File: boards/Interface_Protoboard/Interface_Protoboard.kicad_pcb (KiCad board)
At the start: 2 copper layers, 70 x 70 mm, 385 parts

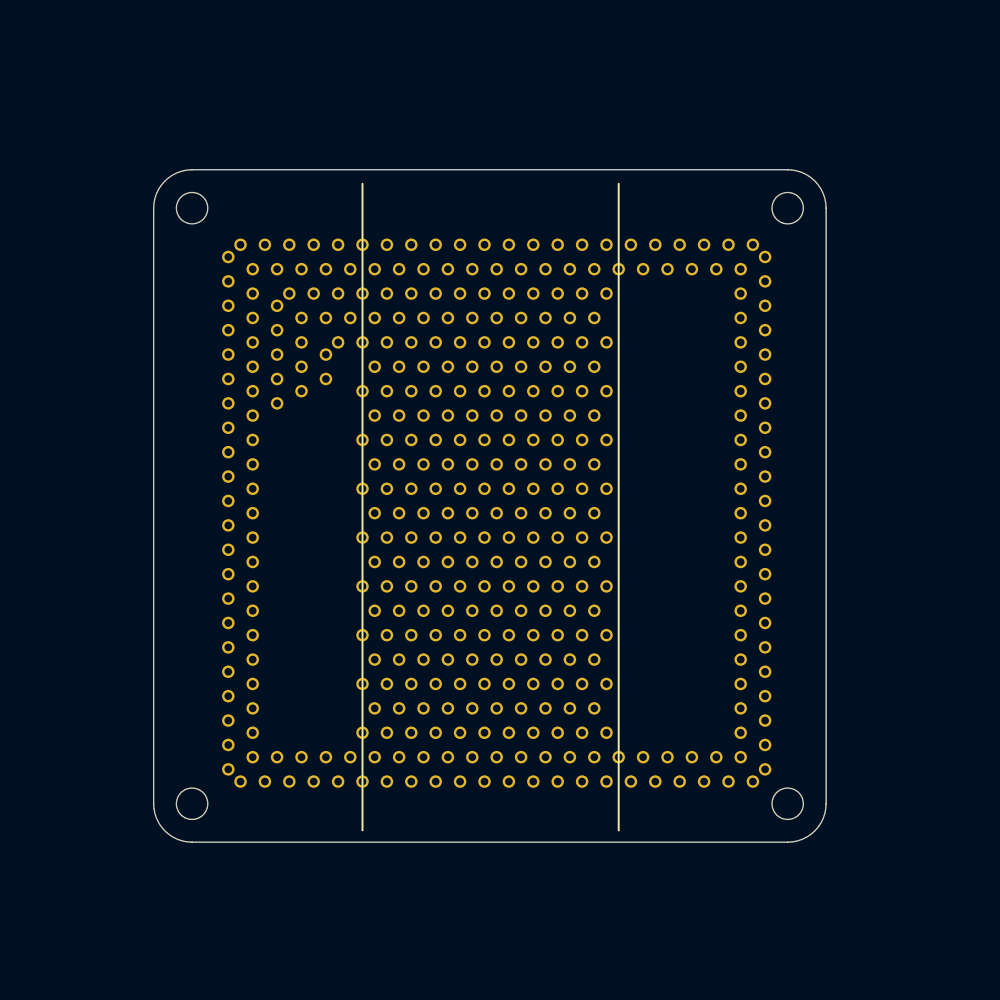
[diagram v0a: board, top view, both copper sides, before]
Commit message: finished interface protoboard and uploaded checked gerbers to drive for ordering
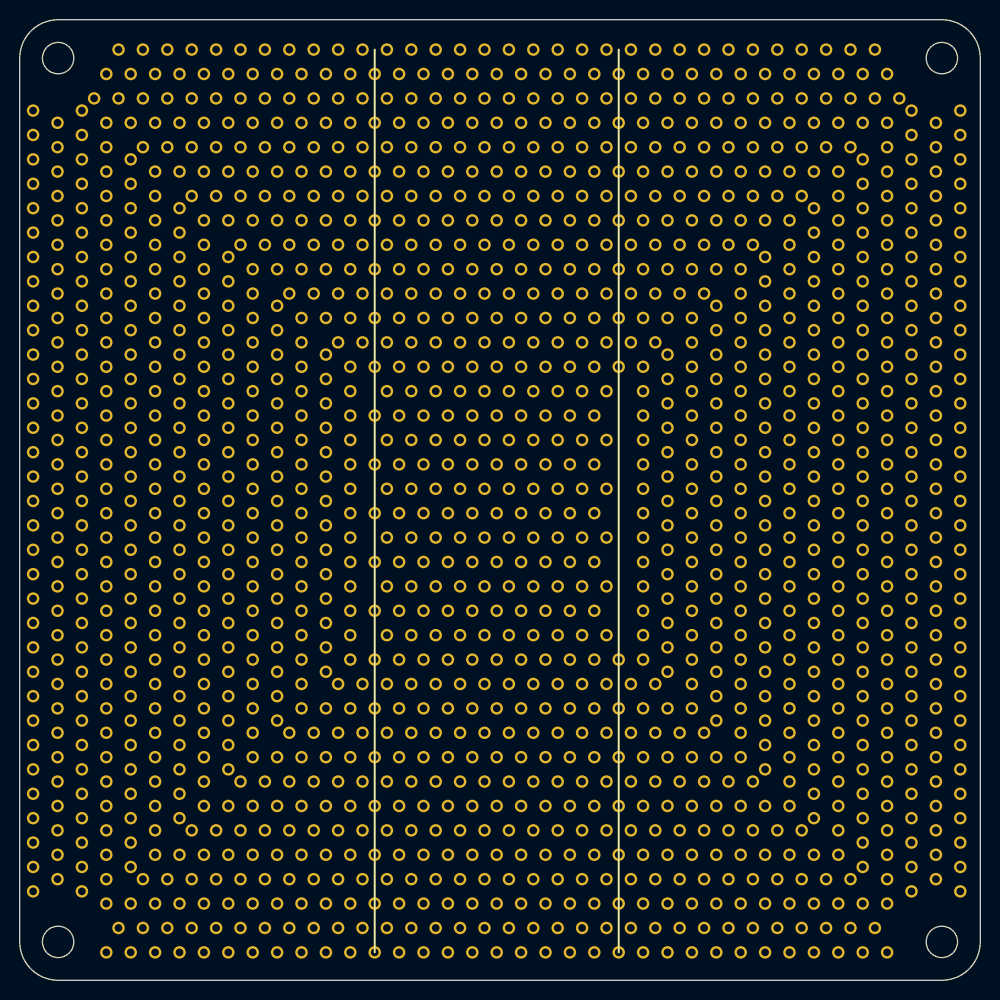
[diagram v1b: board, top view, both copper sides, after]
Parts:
- removed the J? at (138.4, 81.3)
- removed the J? at (138.4, 86.4)
- removed the J? at (138.4, 91.4)
- removed the J? at (138.4, 96.5)
- removed the J? at (138.4, 101.6)
- removed the J? at (138.4, 106.7)
- added J?: micromatch_female_ra_12, footprints:micromatch_via, F.Cu at (137.2, 48.3)
- added J?: micromatch_female_ra_12, footprints:micromatch_via, F.Cu at (139.7, 48.3)
- added J?: micromatch_female_ra_12, footprints:micromatch_via, F.Cu at (142.2, 48.3)
- added J?: micromatch_female_ra_12, footprints:micromatch_via, F.Cu at (144.8, 48.3)
- added J?: micromatch_female_ra_12, footprints:micromatch_via, F.Cu at (147.3, 48.3)
- added J?: micromatch_female_ra_12, footprints:micromatch_via, F.Cu at (149.9, 48.3)
- added J?: micromatch_female_ra_12, footprints:micromatch_via, F.Cu at (152.4, 48.3)
- added J?: micromatch_female_ra_12, footprints:micromatch_via, F.Cu at (154.9, 48.3)
- added J?: micromatch_female_ra_12, footprints:micromatch_via, F.Cu at (157.5, 48.3)
- added J?: micromatch_female_ra_12, footprints:micromatch_via, F.Cu at (160.0, 48.3)
- added J?: micromatch_female_ra_12, footprints:micromatch_via, F.Cu at (162.6, 48.3)
- added J?: micromatch_female_ra_12, footprints:micromatch_via, F.Cu at (165.1, 48.3)
- added J?: micromatch_female_ra_12, footprints:micromatch_via, F.Cu at (167.6, 48.3)
- added J?: micromatch_female_ra_12, footprints:micromatch_via, F.Cu at (170.2, 48.3)
- added J?: micromatch_female_ra_12, footprints:micromatch_via, F.Cu at (172.7, 48.3)
- added J?: micromatch_female_ra_12, footprints:micromatch_via, F.Cu at (175.3, 48.3)
- added J?: micromatch_female_ra_12, footprints:micromatch_via, F.Cu at (177.8, 48.3)
- added J?: micromatch_female_ra_12, footprints:micromatch_via, F.Cu at (180.3, 48.3)
- added J?: micromatch_female_ra_12, footprints:micromatch_via, F.Cu at (182.9, 48.3)
- added J?: micromatch_female_ra_12, footprints:micromatch_via, F.Cu at (185.4, 48.3)
- added J?: micromatch_female_ra_12, footprints:micromatch_via, F.Cu at (188.0, 48.3)
- added J?: micromatch_female_ra_12, footprints:micromatch_via, F.Cu at (190.5, 48.3)
- added J?: micromatch_female_ra_12, footprints:micromatch_via, F.Cu at (193.0, 48.3)
- added J?: micromatch_female_ra_12, footprints:micromatch_via, F.Cu at (191.8, 45.7)
- added J?: micromatch_female_ra_12, footprints:micromatch_via, F.Cu at (189.2, 45.7)
- added J?: micromatch_female_ra_12, footprints:micromatch_via, F.Cu at (186.7, 45.7)
- added J?: micromatch_female_ra_12, footprints:micromatch_via, F.Cu at (184.2, 45.7)
- added J?: micromatch_female_ra_12, footprints:micromatch_via, F.Cu at (181.6, 45.7)
- added J?: micromatch_female_ra_12, footprints:micromatch_via, F.Cu at (179.1, 45.7)
- added J?: micromatch_female_ra_12, footprints:micromatch_via, F.Cu at (176.5, 45.7)
- added J?: micromatch_female_ra_12, footprints:micromatch_via, F.Cu at (174.0, 45.7)
- added J?: micromatch_female_ra_12, footprints:micromatch_via, F.Cu at (171.4, 45.7)
- added J?: micromatch_female_ra_12, footprints:micromatch_via, F.Cu at (168.9, 45.7)
- added J?: micromatch_female_ra_12, footprints:micromatch_via, F.Cu at (166.4, 45.7)
- added J?: micromatch_female_ra_12, footprints:micromatch_via, F.Cu at (163.8, 45.7)
- added J?: micromatch_female_ra_12, footprints:micromatch_via, F.Cu at (161.3, 45.7)
- added J?: micromatch_female_ra_12, footprints:micromatch_via, F.Cu at (158.8, 45.7)
- added J?: micromatch_female_ra_12, footprints:micromatch_via, F.Cu at (156.2, 45.7)
- added J?: micromatch_female_ra_12, footprints:micromatch_via, F.Cu at (153.7, 45.7)
- added J?: micromatch_female_ra_12, footprints:micromatch_via, F.Cu at (151.1, 45.7)
- added J?: micromatch_female_ra_12, footprints:micromatch_via, F.Cu at (148.6, 45.7)
- added J?: micromatch_female_ra_12, footprints:micromatch_via, F.Cu at (146.1, 45.7)
- added J?: micromatch_female_ra_12, footprints:micromatch_via, F.Cu at (143.5, 45.7)
- added J?: micromatch_female_ra_12, footprints:micromatch_via, F.Cu at (141.0, 45.7)
- added J?: micromatch_female_ra_12, footprints:micromatch_via, F.Cu at (138.4, 45.7)
- added J?: micromatch_female_ra_12, footprints:micromatch_via, F.Cu at (135.9, 45.7)
- added J?: micromatch_female_ra_12, footprints:micromatch_via, F.Cu at (133.3, 45.7)
- added J?: micromatch_female_ra_12, footprints:micromatch_via, F.Cu at (130.8, 45.7)
- added J?: micromatch_female_ra_12, footprints:micromatch_via, F.Cu at (128.3, 45.7)
- added J?: micromatch_female_ra_12, footprints:micromatch_via, F.Cu at (125.7, 45.7)
- added J?: micromatch_female_ra_12, footprints:micromatch_via, F.Cu at (123.2, 45.7)
- added J?: micromatch_female_ra_12, footprints:micromatch_via, F.Cu at (120.7, 45.7)
- added J?: micromatch_female_ra_12, footprints:micromatch_via, F.Cu at (118.1, 45.7)
- added J?: micromatch_female_ra_12, footprints:micromatch_via, F.Cu at (115.6, 45.7)
- added J?: micromatch_female_ra_12, footprints:micromatch_via, F.Cu at (113.0, 45.7)
- added J?: micromatch_female_ra_12, footprints:micromatch_via, F.Cu at (114.3, 57.1)
- added J?: micromatch_female_ra_12, footprints:micromatch_via, F.Cu at (114.3, 59.7)
- added J?: micromatch_female_ra_12, footprints:micromatch_via, F.Cu at (114.3, 62.2)
- added J?: micromatch_female_ra_12, footprints:micromatch_via, F.Cu at (114.3, 64.8)
- added J?: micromatch_female_ra_12, footprints:micromatch_via, F.Cu at (114.3, 67.3)
- added J?: micromatch_female_ra_12, footprints:micromatch_via, F.Cu at (114.3, 69.8)
- added J?: micromatch_female_ra_12, footprints:micromatch_via, F.Cu at (114.3, 72.4)
- added J?: micromatch_female_ra_12, footprints:micromatch_via, F.Cu at (114.3, 74.9)
- added J?: micromatch_female_ra_12, footprints:micromatch_via, F.Cu at (114.3, 77.5)
- added J?: micromatch_female_ra_12, footprints:micromatch_via, F.Cu at (114.3, 80.0)
- added J?: micromatch_female_ra_12, footprints:micromatch_via, F.Cu at (114.3, 82.5)
- added J?: micromatch_female_ra_12, footprints:micromatch_via, F.Cu at (114.3, 85.1)
- added J?: micromatch_female_ra_12, footprints:micromatch_via, F.Cu at (114.3, 87.6)
- added J?: micromatch_female_ra_12, footprints:micromatch_via, F.Cu at (114.3, 90.2)
- added J?: micromatch_female_ra_12, footprints:micromatch_via, F.Cu at (114.3, 92.7)
- added J?: micromatch_female_ra_12, footprints:micromatch_via, F.Cu at (114.3, 95.2)
- added J?: micromatch_female_ra_12, footprints:micromatch_via, F.Cu at (114.3, 97.8)
- added J?: micromatch_female_ra_12, footprints:micromatch_via, F.Cu at (114.3, 100.3)
- added J?: micromatch_female_ra_12, footprints:micromatch_via, F.Cu at (114.3, 102.9)
- added J?: micromatch_female_ra_12, footprints:micromatch_via, F.Cu at (114.3, 105.4)
- added J?: micromatch_female_ra_12, footprints:micromatch_via, F.Cu at (114.3, 108.0)
- added J?: micromatch_female_ra_12, footprints:micromatch_via, F.Cu at (114.3, 110.5)
- added J?: micromatch_female_ra_12, footprints:micromatch_via, F.Cu at (114.3, 113.0)
- added J?: micromatch_female_ra_12, footprints:micromatch_via, F.Cu at (114.3, 115.6)
- added J?: micromatch_female_ra_12, footprints:micromatch_via, F.Cu at (114.3, 118.1)
- added J?: micromatch_female_ra_12, footprints:micromatch_via, F.Cu at (114.3, 120.7)
- added J?: micromatch_female_ra_12, footprints:micromatch_via, F.Cu at (114.3, 123.2)
- added J?: micromatch_female_ra_12, footprints:micromatch_via, F.Cu at (114.3, 125.7)
- added J?: micromatch_female_ra_12, footprints:micromatch_via, F.Cu at (114.3, 128.3)
- added J?: micromatch_female_ra_12, footprints:micromatch_via, F.Cu at (114.3, 130.8)
- added J?: micromatch_female_ra_12, footprints:micromatch_via, F.Cu at (111.8, 55.9)
- added J?: micromatch_female_ra_12, footprints:micromatch_via, F.Cu at (111.8, 58.4)
- added J?: micromatch_female_ra_12, footprints:micromatch_via, F.Cu at (111.8, 61.0)
- added J?: micromatch_female_ra_12, footprints:micromatch_via, F.Cu at (111.8, 63.5)
- added J?: micromatch_female_ra_12, footprints:micromatch_via, F.Cu at (111.8, 66.0)
- added J?: micromatch_female_ra_12, footprints:micromatch_via, F.Cu at (111.8, 68.6)
- added J?: micromatch_female_ra_12, footprints:micromatch_via, F.Cu at (111.8, 71.1)
- added J?: micromatch_female_ra_12, footprints:micromatch_via, F.Cu at (111.8, 73.7)
- added J?: micromatch_female_ra_12, footprints:micromatch_via, F.Cu at (111.8, 76.2)
- added J?: micromatch_female_ra_12, footprints:micromatch_via, F.Cu at (111.8, 78.7)
- added J?: micromatch_female_ra_12, footprints:micromatch_via, F.Cu at (111.8, 81.3)
- added J?: micromatch_female_ra_12, footprints:micromatch_via, F.Cu at (111.8, 83.8)
- added J?: micromatch_female_ra_12, footprints:micromatch_via, F.Cu at (111.8, 86.4)
- added J?: micromatch_female_ra_12, footprints:micromatch_via, F.Cu at (111.8, 88.9)
- added J?: micromatch_female_ra_12, footprints:micromatch_via, F.Cu at (111.8, 91.4)
- added J?: micromatch_female_ra_12, footprints:micromatch_via, F.Cu at (111.8, 94.0)
- added J?: micromatch_female_ra_12, footprints:micromatch_via, F.Cu at (111.8, 96.5)
- added J?: micromatch_female_ra_12, footprints:micromatch_via, F.Cu at (111.8, 99.1)
- added J?: micromatch_female_ra_12, footprints:micromatch_via, F.Cu at (111.8, 101.6)
- added J?: micromatch_female_ra_12, footprints:micromatch_via, F.Cu at (111.8, 104.1)
- added J?: micromatch_female_ra_12, footprints:micromatch_via, F.Cu at (111.8, 106.7)
- added J?: micromatch_female_ra_12, footprints:micromatch_via, F.Cu at (111.8, 109.2)
- added J?: micromatch_female_ra_12, footprints:micromatch_via, F.Cu at (111.8, 111.8)
- added J?: micromatch_female_ra_12, footprints:micromatch_via, F.Cu at (111.8, 114.3)
- added J?: micromatch_female_ra_12, footprints:micromatch_via, F.Cu at (111.8, 116.8)
- added J?: micromatch_female_ra_12, footprints:micromatch_via, F.Cu at (111.8, 119.4)
- added J?: micromatch_female_ra_12, footprints:micromatch_via, F.Cu at (111.8, 121.9)
- added J?: micromatch_female_ra_12, footprints:micromatch_via, F.Cu at (111.8, 124.5)
- added J?: micromatch_female_ra_12, footprints:micromatch_via, F.Cu at (111.8, 127.0)
- added J?: micromatch_female_ra_12, footprints:micromatch_via, F.Cu at (111.8, 129.5)
- added J?: micromatch_female_ra_12, footprints:micromatch_via, F.Cu at (111.8, 132.1)
- added J?: micromatch_female_ra_12, footprints:micromatch_via, F.Cu at (111.8, 134.6)
- added J?: micromatch_female_ra_12, footprints:micromatch_via, F.Cu at (109.2, 133.3)
- added J?: micromatch_female_ra_12, footprints:micromatch_via, F.Cu at (109.2, 130.8)
- added J?: micromatch_female_ra_12, footprints:micromatch_via, F.Cu at (109.2, 128.3)
- added J?: micromatch_female_ra_12, footprints:micromatch_via, F.Cu at (109.2, 125.7)
- added J?: micromatch_female_ra_12, footprints:micromatch_via, F.Cu at (109.2, 123.2)
- added J?: micromatch_female_ra_12, footprints:micromatch_via, F.Cu at (109.2, 120.7)
- added J?: micromatch_female_ra_12, footprints:micromatch_via, F.Cu at (109.2, 118.1)
- added J?: micromatch_female_ra_12, footprints:micromatch_via, F.Cu at (109.2, 115.6)
- added J?: micromatch_female_ra_12, footprints:micromatch_via, F.Cu at (109.2, 113.0)
- added J?: micromatch_female_ra_12, footprints:micromatch_via, F.Cu at (109.2, 110.5)
- added J?: micromatch_female_ra_12, footprints:micromatch_via, F.Cu at (109.2, 108.0)
- added J?: micromatch_female_ra_12, footprints:micromatch_via, F.Cu at (109.2, 105.4)
- added J?: micromatch_female_ra_12, footprints:micromatch_via, F.Cu at (109.2, 102.9)
- added J?: micromatch_female_ra_12, footprints:micromatch_via, F.Cu at (109.2, 100.3)
- added J?: micromatch_female_ra_12, footprints:micromatch_via, F.Cu at (109.2, 97.8)
- added J?: micromatch_female_ra_12, footprints:micromatch_via, F.Cu at (109.2, 95.2)
- added J?: micromatch_female_ra_12, footprints:micromatch_via, F.Cu at (109.2, 92.7)
- added J?: micromatch_female_ra_12, footprints:micromatch_via, F.Cu at (109.2, 90.2)
- added J?: micromatch_female_ra_12, footprints:micromatch_via, F.Cu at (109.2, 87.6)
- added J?: micromatch_female_ra_12, footprints:micromatch_via, F.Cu at (109.2, 85.1)
- added J?: micromatch_female_ra_12, footprints:micromatch_via, F.Cu at (109.2, 82.5)
- added J?: micromatch_female_ra_12, footprints:micromatch_via, F.Cu at (109.2, 80.0)
- added J?: micromatch_female_ra_12, footprints:micromatch_via, F.Cu at (109.2, 77.5)
- added J?: micromatch_female_ra_12, footprints:micromatch_via, F.Cu at (109.2, 74.9)
- added J?: micromatch_female_ra_12, footprints:micromatch_via, F.Cu at (109.2, 72.4)
- added J?: micromatch_female_ra_12, footprints:micromatch_via, F.Cu at (109.2, 69.8)
- added J?: micromatch_female_ra_12, footprints:micromatch_via, F.Cu at (109.2, 67.3)
- added J?: micromatch_female_ra_12, footprints:micromatch_via, F.Cu at (109.2, 64.8)
- added J?: micromatch_female_ra_12, footprints:micromatch_via, F.Cu at (109.2, 62.2)
- added J?: micromatch_female_ra_12, footprints:micromatch_via, F.Cu at (109.2, 59.7)
- added J?: micromatch_female_ra_12, footprints:micromatch_via, F.Cu at (109.2, 57.1)
- added J?: micromatch_female_ra_12, footprints:micromatch_via, F.Cu at (109.2, 54.6)
- added J?: micromatch_female_ra_12, footprints:micromatch_via, F.Cu at (106.7, 53.3)
- added J?: micromatch_female_ra_12, footprints:micromatch_via, F.Cu at (106.7, 55.9)
- added J?: micromatch_female_ra_12, footprints:micromatch_via, F.Cu at (106.7, 58.4)
- added J?: micromatch_female_ra_12, footprints:micromatch_via, F.Cu at (106.7, 61.0)
- added J?: micromatch_female_ra_12, footprints:micromatch_via, F.Cu at (106.7, 63.5)
- added J?: micromatch_female_ra_12, footprints:micromatch_via, F.Cu at (104.1, 62.2)
- added J?: micromatch_female_ra_12, footprints:micromatch_via, F.Cu at (104.1, 59.7)
- added J?: micromatch_female_ra_12, footprints:micromatch_via, F.Cu at (104.1, 57.1)
- added J?: micromatch_female_ra_12, footprints:micromatch_via, F.Cu at (104.1, 54.6)
- added J?: micromatch_female_ra_12, footprints:micromatch_via, F.Cu at (104.1, 52.1)
- added J?: micromatch_female_ra_12, footprints:micromatch_via, F.Cu at (104.1, 64.8)
- added J?: micromatch_female_ra_12, footprints:micromatch_via, F.Cu at (104.1, 67.3)
- added J?: micromatch_female_ra_12, footprints:micromatch_via, F.Cu at (104.1, 69.8)
- added J?: micromatch_female_ra_12, footprints:micromatch_via, F.Cu at (104.1, 72.4)
- added J?: micromatch_female_ra_12, footprints:micromatch_via, F.Cu at (104.1, 74.9)
- added J?: micromatch_female_ra_12, footprints:micromatch_via, F.Cu at (104.1, 77.5)
- added J?: micromatch_female_ra_12, footprints:micromatch_via, F.Cu at (104.1, 80.0)
- added J?: micromatch_female_ra_12, footprints:micromatch_via, F.Cu at (104.1, 82.5)
- added J?: micromatch_female_ra_12, footprints:micromatch_via, F.Cu at (106.7, 81.3)
- added J?: micromatch_female_ra_12, footprints:micromatch_via, F.Cu at (106.7, 78.7)
- added J?: micromatch_female_ra_12, footprints:micromatch_via, F.Cu at (106.7, 76.2)
- added J?: micromatch_female_ra_12, footprints:micromatch_via, F.Cu at (106.7, 73.7)
- added J?: micromatch_female_ra_12, footprints:micromatch_via, F.Cu at (106.7, 71.1)
- added J?: micromatch_female_ra_12, footprints:micromatch_via, F.Cu at (106.7, 68.6)
- added J?: micromatch_female_ra_12, footprints:micromatch_via, F.Cu at (106.7, 66.0)
- added J?: micromatch_female_ra_12, footprints:micromatch_via, F.Cu at (106.7, 83.8)
- added J?: micromatch_female_ra_12, footprints:micromatch_via, F.Cu at (106.7, 86.4)
- added J?: micromatch_female_ra_12, footprints:micromatch_via, F.Cu at (106.7, 88.9)
- added J?: micromatch_female_ra_12, footprints:micromatch_via, F.Cu at (106.7, 91.4)
- added J?: micromatch_female_ra_12, footprints:micromatch_via, F.Cu at (106.7, 94.0)
- added J?: micromatch_female_ra_12, footprints:micromatch_via, F.Cu at (106.7, 96.5)
- added J?: micromatch_female_ra_12, footprints:micromatch_via, F.Cu at (106.7, 99.1)
- added J?: micromatch_female_ra_12, footprints:micromatch_via, F.Cu at (106.7, 101.6)
- added J?: micromatch_female_ra_12, footprints:micromatch_via, F.Cu at (104.1, 100.3)
- added J?: micromatch_female_ra_12, footprints:micromatch_via, F.Cu at (104.1, 97.8)
- added J?: micromatch_female_ra_12, footprints:micromatch_via, F.Cu at (104.1, 95.2)
- added J?: micromatch_female_ra_12, footprints:micromatch_via, F.Cu at (104.1, 92.7)
- added J?: micromatch_female_ra_12, footprints:micromatch_via, F.Cu at (104.1, 90.2)
- added J?: micromatch_female_ra_12, footprints:micromatch_via, F.Cu at (104.1, 87.6)
- added J?: micromatch_female_ra_12, footprints:micromatch_via, F.Cu at (104.1, 85.1)
- added J?: micromatch_female_ra_12, footprints:micromatch_via, F.Cu at (104.1, 102.9)
- added J?: micromatch_female_ra_12, footprints:micromatch_via, F.Cu at (104.1, 105.4)
- added J?: micromatch_female_ra_12, footprints:micromatch_via, F.Cu at (104.1, 108.0)
- added J?: micromatch_female_ra_12, footprints:micromatch_via, F.Cu at (104.1, 110.5)
- added J?: micromatch_female_ra_12, footprints:micromatch_via, F.Cu at (104.1, 113.0)
- added J?: micromatch_female_ra_12, footprints:micromatch_via, F.Cu at (104.1, 115.6)
- added J?: micromatch_female_ra_12, footprints:micromatch_via, F.Cu at (104.1, 118.1)
- added J?: micromatch_female_ra_12, footprints:micromatch_via, F.Cu at (106.7, 119.4)
- added J?: micromatch_female_ra_12, footprints:micromatch_via, F.Cu at (106.7, 116.8)
- added J?: micromatch_female_ra_12, footprints:micromatch_via, F.Cu at (106.7, 114.3)
- added J?: micromatch_female_ra_12, footprints:micromatch_via, F.Cu at (106.7, 111.8)
- added J?: micromatch_female_ra_12, footprints:micromatch_via, F.Cu at (106.7, 109.2)
- added J?: micromatch_female_ra_12, footprints:micromatch_via, F.Cu at (106.7, 106.7)
- added J?: micromatch_female_ra_12, footprints:micromatch_via, F.Cu at (106.7, 104.1)
- added J?: micromatch_female_ra_12, footprints:micromatch_via, F.Cu at (106.7, 121.9)
- added J?: micromatch_female_ra_12, footprints:micromatch_via, F.Cu at (106.7, 124.5)
- added J?: micromatch_female_ra_12, footprints:micromatch_via, F.Cu at (106.7, 127.0)
- added J?: micromatch_female_ra_12, footprints:micromatch_via, F.Cu at (106.7, 129.5)
- added J?: micromatch_female_ra_12, footprints:micromatch_via, F.Cu at (106.7, 132.1)
- added J?: micromatch_female_ra_12, footprints:micromatch_via, F.Cu at (104.1, 133.3)
- added J?: micromatch_female_ra_12, footprints:micromatch_via, F.Cu at (104.1, 130.8)
- added J?: micromatch_female_ra_12, footprints:micromatch_via, F.Cu at (104.1, 128.3)
- added J?: micromatch_female_ra_12, footprints:micromatch_via, F.Cu at (104.1, 125.7)
- added J?: micromatch_female_ra_12, footprints:micromatch_via, F.Cu at (104.1, 123.2)
- added J?: micromatch_female_ra_12, footprints:micromatch_via, F.Cu at (104.1, 120.7)
- added J?: micromatch_female_ra_12, footprints:micromatch_via, F.Cu at (114.3, 134.6)
- added J?: micromatch_female_ra_12, footprints:micromatch_via, F.Cu at (116.8, 134.6)
- added J?: micromatch_female_ra_12, footprints:micromatch_via, F.Cu at (119.4, 134.6)
- added J?: micromatch_female_ra_12, footprints:micromatch_via, F.Cu at (121.9, 134.6)
- added J?: micromatch_female_ra_12, footprints:micromatch_via, F.Cu at (124.5, 134.6)
- added J?: micromatch_female_ra_12, footprints:micromatch_via, F.Cu at (127.0, 134.6)
- added J?: micromatch_female_ra_12, footprints:micromatch_via, F.Cu at (129.5, 134.6)
- added J?: micromatch_female_ra_12, footprints:micromatch_via, F.Cu at (132.1, 134.6)
- added J?: micromatch_female_ra_12, footprints:micromatch_via, F.Cu at (134.6, 134.6)
- added J?: micromatch_female_ra_12, footprints:micromatch_via, F.Cu at (137.2, 134.6)
- added J?: micromatch_female_ra_12, footprints:micromatch_via, F.Cu at (139.7, 134.6)
- added J?: micromatch_female_ra_12, footprints:micromatch_via, F.Cu at (142.2, 134.6)
- added J?: micromatch_female_ra_12, footprints:micromatch_via, F.Cu at (144.8, 134.6)
- added J?: micromatch_female_ra_12, footprints:micromatch_via, F.Cu at (147.3, 134.6)
- added J?: micromatch_female_ra_12, footprints:micromatch_via, F.Cu at (146.1, 137.2)
- added J?: micromatch_female_ra_12, footprints:micromatch_via, F.Cu at (143.5, 137.2)
- added J?: micromatch_female_ra_12, footprints:micromatch_via, F.Cu at (141.0, 137.2)
- added J?: micromatch_female_ra_12, footprints:micromatch_via, F.Cu at (138.4, 137.2)
- added J?: micromatch_female_ra_12, footprints:micromatch_via, F.Cu at (135.9, 137.2)
- added J?: micromatch_female_ra_12, footprints:micromatch_via, F.Cu at (133.3, 137.2)
- added J?: micromatch_female_ra_12, footprints:micromatch_via, F.Cu at (130.8, 137.2)
- added J?: micromatch_female_ra_12, footprints:micromatch_via, F.Cu at (128.3, 137.2)
- added J?: micromatch_female_ra_12, footprints:micromatch_via, F.Cu at (125.7, 137.2)
- added J?: micromatch_female_ra_12, footprints:micromatch_via, F.Cu at (123.2, 137.2)
- added J?: micromatch_female_ra_12, footprints:micromatch_via, F.Cu at (120.7, 137.2)
- added J?: micromatch_female_ra_12, footprints:micromatch_via, F.Cu at (118.1, 137.2)
- added J?: micromatch_female_ra_12, footprints:micromatch_via, F.Cu at (115.6, 137.2)
- added J?: micromatch_female_ra_12, footprints:micromatch_via, F.Cu at (113.0, 137.2)
- added J?: micromatch_female_ra_12, footprints:micromatch_via, F.Cu at (111.8, 139.7)
- added J?: micromatch_female_ra_12, footprints:micromatch_via, F.Cu at (114.3, 139.7)
- added J?: micromatch_female_ra_12, footprints:micromatch_via, F.Cu at (116.8, 139.7)
- added J?: micromatch_female_ra_12, footprints:micromatch_via, F.Cu at (119.4, 139.7)
- added J?: micromatch_female_ra_12, footprints:micromatch_via, F.Cu at (121.9, 139.7)
- added J?: micromatch_female_ra_12, footprints:micromatch_via, F.Cu at (124.5, 139.7)
- added J?: micromatch_female_ra_12, footprints:micromatch_via, F.Cu at (127.0, 139.7)
- added J?: micromatch_female_ra_12, footprints:micromatch_via, F.Cu at (129.5, 139.7)
- added J?: micromatch_female_ra_12, footprints:micromatch_via, F.Cu at (132.1, 139.7)
- added J?: micromatch_female_ra_12, footprints:micromatch_via, F.Cu at (134.6, 139.7)
- added J?: micromatch_female_ra_12, footprints:micromatch_via, F.Cu at (137.2, 139.7)
- added J?: micromatch_female_ra_12, footprints:micromatch_via, F.Cu at (139.7, 139.7)
- added J?: micromatch_female_ra_12, footprints:micromatch_via, F.Cu at (142.2, 139.7)
- added J?: micromatch_female_ra_12, footprints:micromatch_via, F.Cu at (144.8, 139.7)
- added J?: micromatch_female_ra_12, footprints:micromatch_via, F.Cu at (147.3, 139.7)
- added J?: micromatch_female_ra_12, footprints:micromatch_via, F.Cu at (149.9, 134.6)
- added J?: micromatch_female_ra_12, footprints:micromatch_via, F.Cu at (152.4, 134.6)
- added J?: micromatch_female_ra_12, footprints:micromatch_via, F.Cu at (154.9, 134.6)
- added J?: micromatch_female_ra_12, footprints:micromatch_via, F.Cu at (157.5, 134.6)
- added J?: micromatch_female_ra_12, footprints:micromatch_via, F.Cu at (160.0, 134.6)
- added J?: micromatch_female_ra_12, footprints:micromatch_via, F.Cu at (162.6, 134.6)
- added J?: micromatch_female_ra_12, footprints:micromatch_via, F.Cu at (165.1, 134.6)
- added J?: micromatch_female_ra_12, footprints:micromatch_via, F.Cu at (167.6, 134.6)
- added J?: micromatch_female_ra_12, footprints:micromatch_via, F.Cu at (170.2, 134.6)
- added J?: micromatch_female_ra_12, footprints:micromatch_via, F.Cu at (172.7, 134.6)
- added J?: micromatch_female_ra_12, footprints:micromatch_via, F.Cu at (175.3, 134.6)
- added J?: micromatch_female_ra_12, footprints:micromatch_via, F.Cu at (177.8, 134.6)
- added J?: micromatch_female_ra_12, footprints:micromatch_via, F.Cu at (180.3, 134.6)
- added J?: micromatch_female_ra_12, footprints:micromatch_via, F.Cu at (182.9, 134.6)
- added J?: micromatch_female_ra_12, footprints:micromatch_via, F.Cu at (185.4, 134.6)
- added J?: micromatch_female_ra_12, footprints:micromatch_via, F.Cu at (188.0, 134.6)
- added J?: micromatch_female_ra_12, footprints:micromatch_via, F.Cu at (190.5, 134.6)
- added J?: micromatch_female_ra_12, footprints:micromatch_via, F.Cu at (193.0, 134.6)
- added J?: micromatch_female_ra_12, footprints:micromatch_via, F.Cu at (191.8, 137.2)
- added J?: micromatch_female_ra_12, footprints:micromatch_via, F.Cu at (189.2, 137.2)
- added J?: micromatch_female_ra_12, footprints:micromatch_via, F.Cu at (186.7, 137.2)
- added J?: micromatch_female_ra_12, footprints:micromatch_via, F.Cu at (184.2, 137.2)
- added J?: micromatch_female_ra_12, footprints:micromatch_via, F.Cu at (181.6, 137.2)
- added J?: micromatch_female_ra_12, footprints:micromatch_via, F.Cu at (179.1, 137.2)
- added J?: micromatch_female_ra_12, footprints:micromatch_via, F.Cu at (176.5, 137.2)
- added J?: micromatch_female_ra_12, footprints:micromatch_via, F.Cu at (174.0, 137.2)
- added J?: micromatch_female_ra_12, footprints:micromatch_via, F.Cu at (171.4, 137.2)
- added J?: micromatch_female_ra_12, footprints:micromatch_via, F.Cu at (168.9, 137.2)
- added J?: micromatch_female_ra_12, footprints:micromatch_via, F.Cu at (166.4, 137.2)
- added J?: micromatch_female_ra_12, footprints:micromatch_via, F.Cu at (163.8, 137.2)
- added J?: micromatch_female_ra_12, footprints:micromatch_via, F.Cu at (161.3, 137.2)
- added J?: micromatch_female_ra_12, footprints:micromatch_via, F.Cu at (158.8, 137.2)
- added J?: micromatch_female_ra_12, footprints:micromatch_via, F.Cu at (156.2, 137.2)
- added J?: micromatch_female_ra_12, footprints:micromatch_via, F.Cu at (153.7, 137.2)
- added J?: micromatch_female_ra_12, footprints:micromatch_via, F.Cu at (151.1, 137.2)
- added J?: micromatch_female_ra_12, footprints:micromatch_via, F.Cu at (148.6, 137.2)
- added J?: micromatch_female_ra_12, footprints:micromatch_via, F.Cu at (149.9, 139.7)
- added J?: micromatch_female_ra_12, footprints:micromatch_via, F.Cu at (152.4, 139.7)
- added J?: micromatch_female_ra_12, footprints:micromatch_via, F.Cu at (154.9, 139.7)
- added J?: micromatch_female_ra_12, footprints:micromatch_via, F.Cu at (157.5, 139.7)
- added J?: micromatch_female_ra_12, footprints:micromatch_via, F.Cu at (160.0, 139.7)
- added J?: micromatch_female_ra_12, footprints:micromatch_via, F.Cu at (162.6, 139.7)
- added J?: micromatch_female_ra_12, footprints:micromatch_via, F.Cu at (165.1, 139.7)
- added J?: micromatch_female_ra_12, footprints:micromatch_via, F.Cu at (167.6, 139.7)
- added J?: micromatch_female_ra_12, footprints:micromatch_via, F.Cu at (170.2, 139.7)
- added J?: micromatch_female_ra_12, footprints:micromatch_via, F.Cu at (172.7, 139.7)
- added J?: micromatch_female_ra_12, footprints:micromatch_via, F.Cu at (175.3, 139.7)
- added J?: micromatch_female_ra_12, footprints:micromatch_via, F.Cu at (177.8, 139.7)
- added J?: micromatch_female_ra_12, footprints:micromatch_via, F.Cu at (180.3, 139.7)
- added J?: micromatch_female_ra_12, footprints:micromatch_via, F.Cu at (182.9, 139.7)
- added J?: micromatch_female_ra_12, footprints:micromatch_via, F.Cu at (185.4, 139.7)
- added J?: micromatch_female_ra_12, footprints:micromatch_via, F.Cu at (188.0, 139.7)
- added J?: micromatch_female_ra_12, footprints:micromatch_via, F.Cu at (190.5, 139.7)
- added J?: micromatch_female_ra_12, footprints:micromatch_via, F.Cu at (193.0, 139.7)
- added J?: micromatch_female_ra_12, footprints:micromatch_via, F.Cu at (193.0, 132.1)
- added J?: micromatch_female_ra_12, footprints:micromatch_via, F.Cu at (193.0, 129.5)
- added J?: micromatch_female_ra_12, footprints:micromatch_via, F.Cu at (193.0, 127.0)
- added J?: micromatch_female_ra_12, footprints:micromatch_via, F.Cu at (193.0, 124.5)
- added J?: micromatch_female_ra_12, footprints:micromatch_via, F.Cu at (193.0, 121.9)
- added J?: micromatch_female_ra_12, footprints:micromatch_via, F.Cu at (193.0, 119.4)
- added J?: micromatch_female_ra_12, footprints:micromatch_via, F.Cu at (195.6, 120.7)
- added J?: micromatch_female_ra_12, footprints:micromatch_via, F.Cu at (195.6, 123.2)
- added J?: micromatch_female_ra_12, footprints:micromatch_via, F.Cu at (195.6, 125.7)
- added J?: micromatch_female_ra_12, footprints:micromatch_via, F.Cu at (195.6, 128.3)
- added J?: micromatch_female_ra_12, footprints:micromatch_via, F.Cu at (195.6, 130.8)
- added J?: micromatch_female_ra_12, footprints:micromatch_via, F.Cu at (195.6, 133.3)
- added J?: micromatch_female_ra_12, footprints:micromatch_via, F.Cu at (198.1, 132.1)
- added J?: micromatch_female_ra_12, footprints:micromatch_via, F.Cu at (198.1, 129.5)
- added J?: micromatch_female_ra_12, footprints:micromatch_via, F.Cu at (198.1, 127.0)
- added J?: micromatch_female_ra_12, footprints:micromatch_via, F.Cu at (198.1, 124.5)
- added J?: micromatch_female_ra_12, footprints:micromatch_via, F.Cu at (198.1, 121.9)
- added J?: micromatch_female_ra_12, footprints:micromatch_via, F.Cu at (198.1, 119.4)
- added J?: micromatch_female_ra_12, footprints:micromatch_via, F.Cu at (200.7, 120.7)
- added J?: micromatch_female_ra_12, footprints:micromatch_via, F.Cu at (200.7, 123.2)
- added J?: micromatch_female_ra_12, footprints:micromatch_via, F.Cu at (200.7, 125.7)
- added J?: micromatch_female_ra_12, footprints:micromatch_via, F.Cu at (200.7, 128.3)
- added J?: micromatch_female_ra_12, footprints:micromatch_via, F.Cu at (200.7, 130.8)
- added J?: micromatch_female_ra_12, footprints:micromatch_via, F.Cu at (200.7, 133.3)
- added J?: micromatch_female_ra_12, footprints:micromatch_via, F.Cu at (193.0, 116.8)
- added J?: micromatch_female_ra_12, footprints:micromatch_via, F.Cu at (193.0, 114.3)
- added J?: micromatch_female_ra_12, footprints:micromatch_via, F.Cu at (193.0, 111.8)
- added J?: micromatch_female_ra_12, footprints:micromatch_via, F.Cu at (193.0, 109.2)
- added J?: micromatch_female_ra_12, footprints:micromatch_via, F.Cu at (193.0, 106.7)
- added J?: micromatch_female_ra_12, footprints:micromatch_via, F.Cu at (193.0, 104.1)
- added J?: micromatch_female_ra_12, footprints:micromatch_via, F.Cu at (193.0, 101.6)
- added J?: micromatch_female_ra_12, footprints:micromatch_via, F.Cu at (193.0, 99.1)
- added J?: micromatch_female_ra_12, footprints:micromatch_via, F.Cu at (193.0, 96.5)
- added J?: micromatch_female_ra_12, footprints:micromatch_via, F.Cu at (193.0, 94.0)
- added J?: micromatch_female_ra_12, footprints:micromatch_via, F.Cu at (195.6, 92.7)
- added J?: micromatch_female_ra_12, footprints:micromatch_via, F.Cu at (195.6, 95.2)
- added J?: micromatch_female_ra_12, footprints:micromatch_via, F.Cu at (195.6, 97.8)
- added J?: micromatch_female_ra_12, footprints:micromatch_via, F.Cu at (195.6, 100.3)
- added J?: micromatch_female_ra_12, footprints:micromatch_via, F.Cu at (195.6, 102.9)
- added J?: micromatch_female_ra_12, footprints:micromatch_via, F.Cu at (195.6, 105.4)
- added J?: micromatch_female_ra_12, footprints:micromatch_via, F.Cu at (195.6, 108.0)
- added J?: micromatch_female_ra_12, footprints:micromatch_via, F.Cu at (195.6, 110.5)
- added J?: micromatch_female_ra_12, footprints:micromatch_via, F.Cu at (195.6, 113.0)
- added J?: micromatch_female_ra_12, footprints:micromatch_via, F.Cu at (195.6, 115.6)
- added J?: micromatch_female_ra_12, footprints:micromatch_via, F.Cu at (195.6, 118.1)
- added J?: micromatch_female_ra_12, footprints:micromatch_via, F.Cu at (198.1, 116.8)
- added J?: micromatch_female_ra_12, footprints:micromatch_via, F.Cu at (198.1, 114.3)
- added J?: micromatch_female_ra_12, footprints:micromatch_via, F.Cu at (198.1, 111.8)
- added J?: micromatch_female_ra_12, footprints:micromatch_via, F.Cu at (198.1, 109.2)
- added J?: micromatch_female_ra_12, footprints:micromatch_via, F.Cu at (198.1, 106.7)
- added J?: micromatch_female_ra_12, footprints:micromatch_via, F.Cu at (198.1, 104.1)
- added J?: micromatch_female_ra_12, footprints:micromatch_via, F.Cu at (198.1, 101.6)
- added J?: micromatch_female_ra_12, footprints:micromatch_via, F.Cu at (198.1, 99.1)
- added J?: micromatch_female_ra_12, footprints:micromatch_via, F.Cu at (200.7, 97.8)
- added J?: micromatch_female_ra_12, footprints:micromatch_via, F.Cu at (200.7, 100.3)
- added J?: micromatch_female_ra_12, footprints:micromatch_via, F.Cu at (200.7, 102.9)
- added J?: micromatch_female_ra_12, footprints:micromatch_via, F.Cu at (200.7, 105.4)
- added J?: micromatch_female_ra_12, footprints:micromatch_via, F.Cu at (200.7, 108.0)
- added J?: micromatch_female_ra_12, footprints:micromatch_via, F.Cu at (200.7, 110.5)
- added J?: micromatch_female_ra_12, footprints:micromatch_via, F.Cu at (200.7, 113.0)
- added J?: micromatch_female_ra_12, footprints:micromatch_via, F.Cu at (200.7, 115.6)
- added J?: micromatch_female_ra_12, footprints:micromatch_via, F.Cu at (200.7, 118.1)
- added J?: micromatch_female_ra_12, footprints:micromatch_via, F.Cu at (198.1, 96.5)
- added J?: micromatch_female_ra_12, footprints:micromatch_via, F.Cu at (198.1, 94.0)
- added J?: micromatch_female_ra_12, footprints:micromatch_via, F.Cu at (198.1, 91.4)
- added J?: micromatch_female_ra_12, footprints:micromatch_via, F.Cu at (198.1, 88.9)
- added J?: micromatch_female_ra_12, footprints:micromatch_via, F.Cu at (198.1, 86.4)
- added J?: micromatch_female_ra_12, footprints:micromatch_via, F.Cu at (198.1, 83.8)
- added J?: micromatch_female_ra_12, footprints:micromatch_via, F.Cu at (198.1, 81.3)
- added J?: micromatch_female_ra_12, footprints:micromatch_via, F.Cu at (198.1, 78.7)
- added J?: micromatch_female_ra_12, footprints:micromatch_via, F.Cu at (198.1, 76.2)
- added J?: micromatch_female_ra_12, footprints:micromatch_via, F.Cu at (200.7, 74.9)
- added J?: micromatch_female_ra_12, footprints:micromatch_via, F.Cu at (200.7, 77.5)
- added J?: micromatch_female_ra_12, footprints:micromatch_via, F.Cu at (200.7, 80.0)
- added J?: micromatch_female_ra_12, footprints:micromatch_via, F.Cu at (200.7, 82.5)
- added J?: micromatch_female_ra_12, footprints:micromatch_via, F.Cu at (200.7, 85.1)
- added J?: micromatch_female_ra_12, footprints:micromatch_via, F.Cu at (200.7, 87.6)
- added J?: micromatch_female_ra_12, footprints:micromatch_via, F.Cu at (200.7, 90.2)
- added J?: micromatch_female_ra_12, footprints:micromatch_via, F.Cu at (200.7, 92.7)
- added J?: micromatch_female_ra_12, footprints:micromatch_via, F.Cu at (200.7, 95.2)
- added J?: micromatch_female_ra_12, footprints:micromatch_via, F.Cu at (193.0, 91.4)
- added J?: micromatch_female_ra_12, footprints:micromatch_via, F.Cu at (193.0, 88.9)
- added J?: micromatch_female_ra_12, footprints:micromatch_via, F.Cu at (193.0, 86.4)
- added J?: micromatch_female_ra_12, footprints:micromatch_via, F.Cu at (193.0, 83.8)
- added J?: micromatch_female_ra_12, footprints:micromatch_via, F.Cu at (193.0, 81.3)
- added J?: micromatch_female_ra_12, footprints:micromatch_via, F.Cu at (193.0, 78.7)
- added J?: micromatch_female_ra_12, footprints:micromatch_via, F.Cu at (193.0, 76.2)
- added J?: micromatch_female_ra_12, footprints:micromatch_via, F.Cu at (195.6, 74.9)
- added J?: micromatch_female_ra_12, footprints:micromatch_via, F.Cu at (195.6, 77.5)
- added J?: micromatch_female_ra_12, footprints:micromatch_via, F.Cu at (195.6, 80.0)
- added J?: micromatch_female_ra_12, footprints:micromatch_via, F.Cu at (195.6, 82.5)
- added J?: micromatch_female_ra_12, footprints:micromatch_via, F.Cu at (195.6, 85.1)
- added J?: micromatch_female_ra_12, footprints:micromatch_via, F.Cu at (195.6, 87.6)
- added J?: micromatch_female_ra_12, footprints:micromatch_via, F.Cu at (195.6, 90.2)
- added J?: micromatch_female_ra_12, footprints:micromatch_via, F.Cu at (193.0, 73.7)
- added J?: micromatch_female_ra_12, footprints:micromatch_via, F.Cu at (193.0, 71.1)
- added J?: micromatch_female_ra_12, footprints:micromatch_via, F.Cu at (193.0, 68.6)
- added J?: micromatch_female_ra_12, footprints:micromatch_via, F.Cu at (193.0, 66.0)
- added J?: micromatch_female_ra_12, footprints:micromatch_via, F.Cu at (193.0, 63.5)
- added J?: micromatch_female_ra_12, footprints:micromatch_via, F.Cu at (193.0, 61.0)
- added J?: micromatch_female_ra_12, footprints:micromatch_via, F.Cu at (193.0, 58.4)
- added J?: micromatch_female_ra_12, footprints:micromatch_via, F.Cu at (193.0, 55.9)
- added J?: micromatch_female_ra_12, footprints:micromatch_via, F.Cu at (195.6, 54.6)
- added J?: micromatch_female_ra_12, footprints:micromatch_via, F.Cu at (195.6, 57.1)
- added J?: micromatch_female_ra_12, footprints:micromatch_via, F.Cu at (195.6, 59.7)
- added J?: micromatch_female_ra_12, footprints:micromatch_via, F.Cu at (195.6, 62.2)
- added J?: micromatch_female_ra_12, footprints:micromatch_via, F.Cu at (195.6, 64.8)
- added J?: micromatch_female_ra_12, footprints:micromatch_via, F.Cu at (195.6, 67.3)
- added J?: micromatch_female_ra_12, footprints:micromatch_via, F.Cu at (195.6, 69.8)
- added J?: micromatch_female_ra_12, footprints:micromatch_via, F.Cu at (195.6, 72.4)
- added J?: micromatch_female_ra_12, footprints:micromatch_via, F.Cu at (198.1, 73.7)
- added J?: micromatch_female_ra_12, footprints:micromatch_via, F.Cu at (198.1, 71.1)
- added J?: micromatch_female_ra_12, footprints:micromatch_via, F.Cu at (198.1, 68.6)
- added J?: micromatch_female_ra_12, footprints:micromatch_via, F.Cu at (198.1, 66.0)
- added J?: micromatch_female_ra_12, footprints:micromatch_via, F.Cu at (198.1, 63.5)
- added J?: micromatch_female_ra_12, footprints:micromatch_via, F.Cu at (198.1, 61.0)
- added J?: micromatch_female_ra_12, footprints:micromatch_via, F.Cu at (198.1, 58.4)
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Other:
- board size 70 x 70 mm -> 100 x 100 mm
